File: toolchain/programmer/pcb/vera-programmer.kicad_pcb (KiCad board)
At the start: 2 copper layers, 43.2 x 67.3 mm, 8 parts, among them J1 Conn_02x05_Odd_Even, SW1 SW_Push, U1 Pico

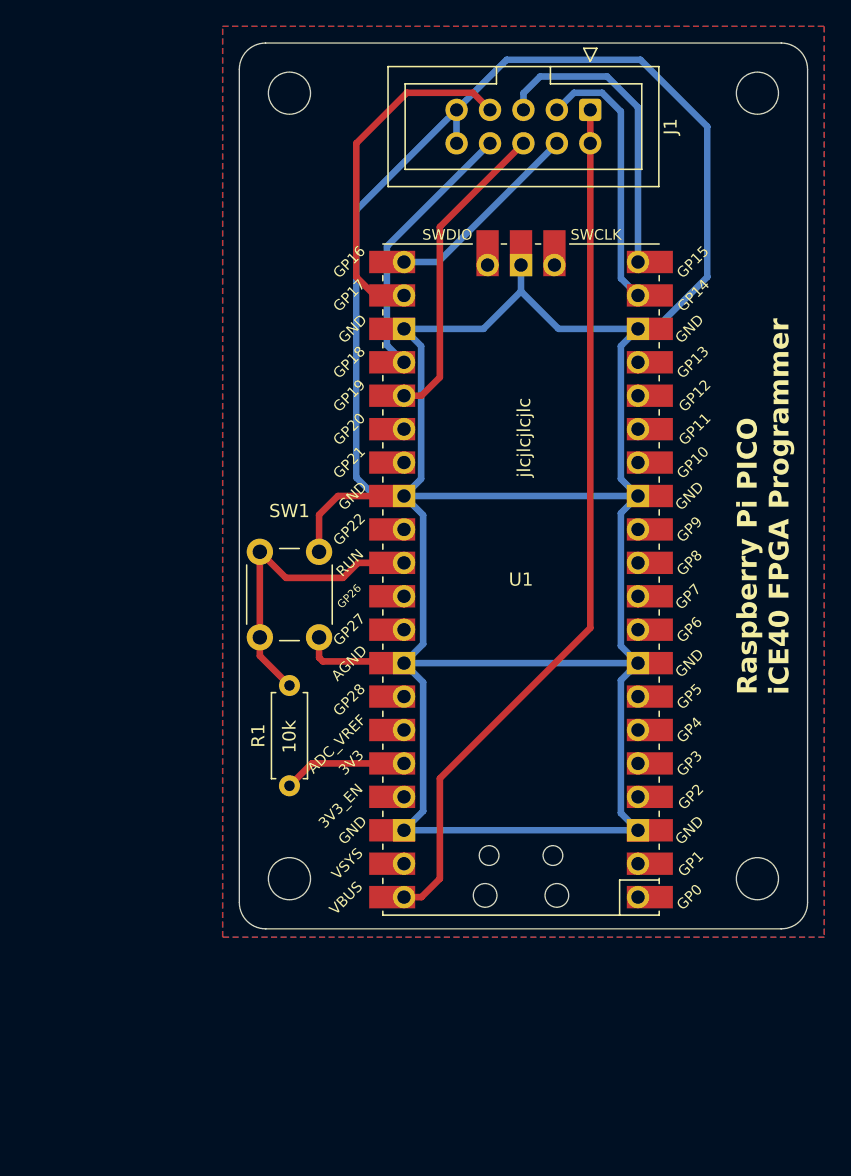
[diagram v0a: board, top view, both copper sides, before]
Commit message: Fixing programmer board and updating licensing
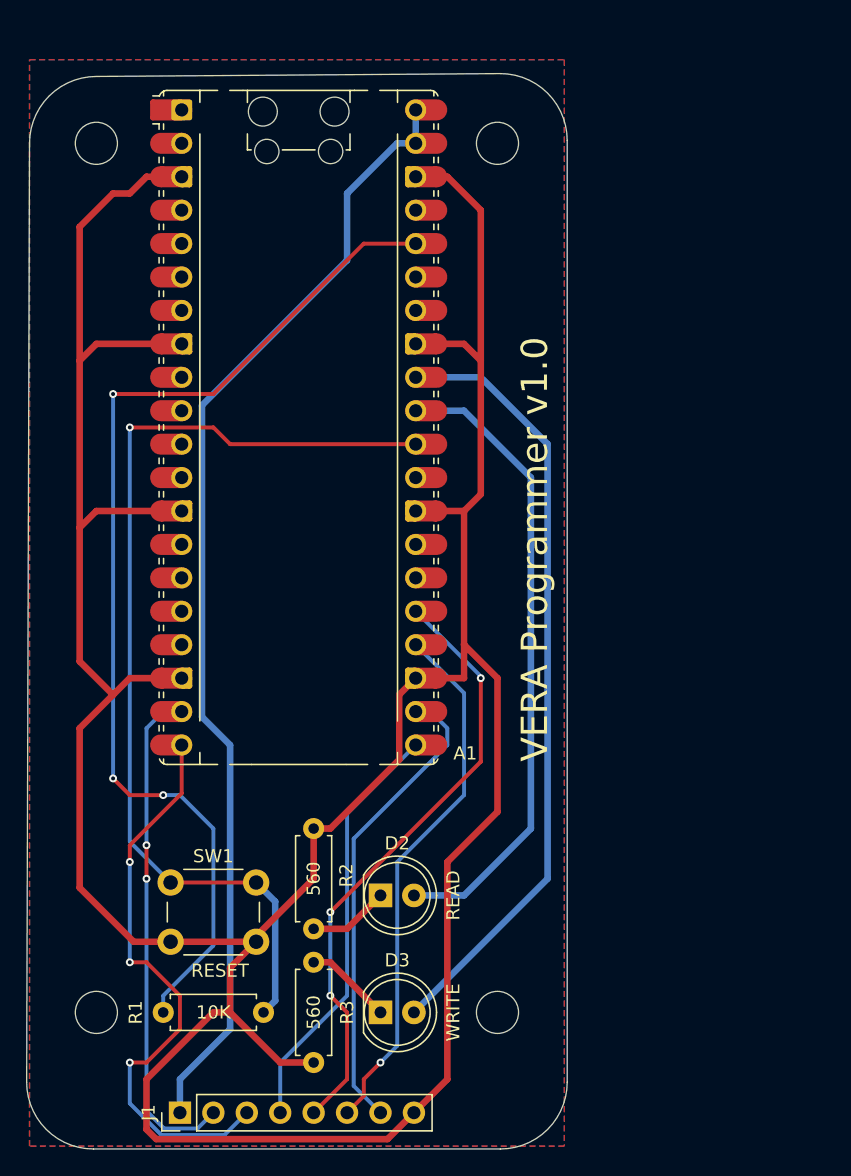
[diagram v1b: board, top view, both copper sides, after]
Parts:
- removed U1: Pico, MCU_RaspberryPi_and_Boards:RPi_Pico_SMD_TH
- added A1: RaspberryPi_Pico, Module:RaspberryPi_Pico_Common_Unspecified, F.Cu at (38.8, 64.8)
- added D2: READ, LED_THT:LED_D5.0mm, F.Cu at (45.0, 100.3)
- added D3: WRITE, LED_THT:LED_D5.0mm, F.Cu at (45.0, 109.2)
- added R2: 560, Resistor_THT:R_Axial_DIN0207_L6.3mm_D2.5mm_P7.62mm_Horizontal, F.Cu at (39.9, 102.9)
- added R3: 560, Resistor_THT:R_Axial_DIN0207_L6.3mm_D2.5mm_P7.62mm_Horizontal, F.Cu at (39.9, 105.4)
- H1, H2, H3, H4: footprint MountingHole:MountingHole_3.2mm_M3_DIN965 -> MountingHole:MountingHole_3.2mm_M3
- J1: value Conn_02x05_Odd_Even -> Prog; footprint Connector_IDC:IDC-Header_2x05_P2.54mm_Vertical -> Connector_PinHeader_2.54mm:PinHeader_1x08_P2.54mm_Vertical
- R1: value 10k -> 10K
- SW1: value SW_Push -> RESET
- moved J1 82.3 mm to (29.8, 116.8), turned to 90 degrees
- moved H4 72.6 mm to (53.9, 109.2)
- moved H3 71.4 mm to (23.4, 109.2)
- moved H2 59.3 mm to (53.9, 43.2)
- moved H1 57.8 mm to (23.4, 43.2)
- moved SW1 19.8 mm to (29.1, 99.3), turned to 0 degrees
- moved R1 19.7 mm to (28.5, 109.2), turned to 0 degrees
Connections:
- J1 pad 2: +5V -> FPGA_CDONE
- J1 pad 3: FPGA_CDONE -> FPGA_CRESET_B
- J1 pad 5: FPGA_CRESET_B -> SPI_MOSI
- J1 pad 6: SPI_MOSI -> SPI_SCK
- J1 pad 8: SPI_SCK -> GND
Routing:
- net +3V3: track 9.41 -> 81.7 mm, vias 0 -> 3
- net GPIO27_3v3: track 0.00 -> 59.5 mm
- net RUN: track 23.3 -> 75.5 mm, vias 0 -> 1
- net GPIO26_3v3: track 0.00 -> 48.5 mm
- net SPI_MOSI: track 23.7 -> 46.5 mm, vias 0 -> 3
- net FPGA_CRESET_B: track 23.2 -> 44.1 mm, vias 0 -> 3
- net SPI_SCK: track 20.4 -> 40.8 mm, vias 0 -> 1
- net +5V: track 66.5 -> 86.2 mm
- net FPGA_CDONE: track 20.5 -> 38.4 mm, vias 0 -> 2
- net SPI_MISO: track 15.4 -> 32.2 mm
- net SPI_SSEL_N: track 26.7 -> 35.9 mm
- net GND: track 255.3 -> 262.1 mm
- net Net-(D3-K): track 0.00 -> 6.66 mm
- net Net-(D2-K): track 0.00 -> 6.13 mm
- added copper zone on B.Cu, net +5V
- removed copper zone on B.Cu, net GND
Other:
- board size 43.2 x 67.3 mm -> 41.1 x 81.7 mm
- board text added: "VERA Programmer v1.0"
- board text removed: "Raspberry Pi PICO iCE40 FPGA Programmer"
- board text removed: "jlcjlcjlcjlc"
